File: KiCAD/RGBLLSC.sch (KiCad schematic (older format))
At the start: 16 parts, among them P1 PICKIT3, P2 RGB-LED-Strip, Q1 FQP30N06L, Q2 FQP30N06L, Q3 FQP30N06L, U1 PIC12F1840

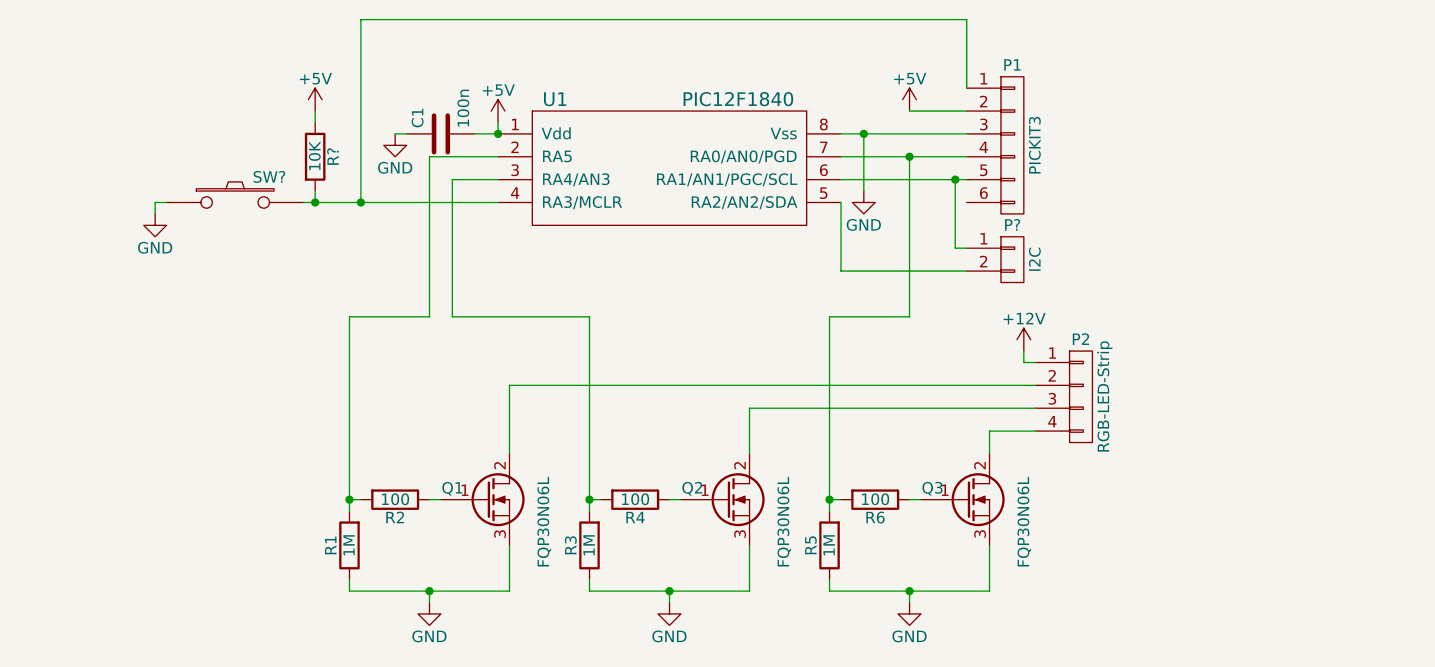
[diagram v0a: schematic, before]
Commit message: Updated Schematic
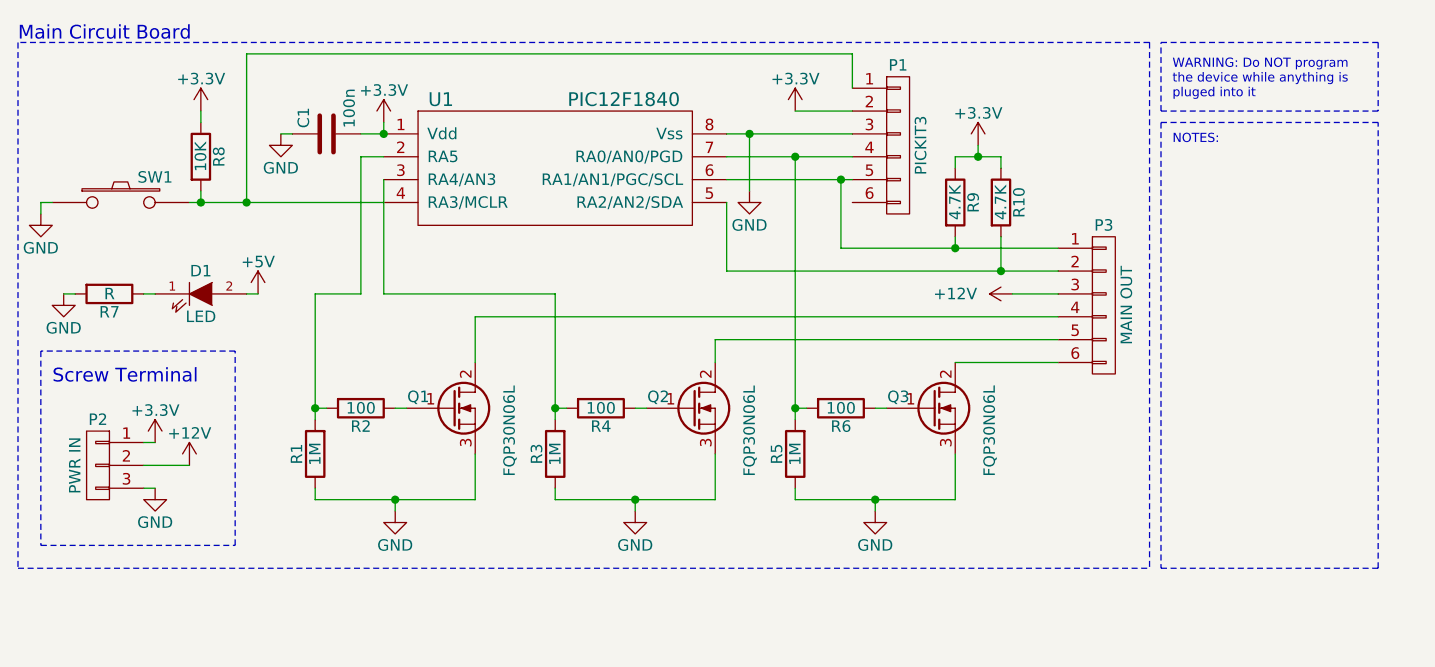
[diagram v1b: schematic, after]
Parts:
- removed P2: RGB-LED-Strip, symbol CONN_01X04
- removed P?: I2C, symbol CONN_01X02
- added D1: LED, symbol LED
- added P2: PWR IN, symbol CONN_01X03
- added P3: MAIN OUT, symbol CONN_01X06
- added R10, R9: 4.7K, symbol R
- added R7: R, symbol R
- gave numbers to parts that had none: 2
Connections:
- net +12V: now also P2.2 (P2), P3.3 (P3)
- net +5V: now also D1.2 (A); no longer C1.2, P1.2 (P2), R8.1, U1.1 (Vdd)
- net GND: now also P2.3 (P3), R7.2
- net at Q2.2 (D): now also P3.5 (P5)
- net at U1.5 (RA2/AN2/SDA): now also P3.2 (P2), R10.2
- net at P1.5 (P5), U1.6 (RA1/AN1/PGC/SCL): now also P3.1 (P1), R9.2
- net at Q1.2 (D): now also P3.4 (P4)
- net at Q3.2 (D): now also P3.6 (P6)
- new net: D1.1 (K), R7.1
- new net +3V3: C1.2, P1.2 (P2), P2.1 (P1), R10.1, R8.1, R9.1, U1.1 (Vdd)
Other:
- note added: "Main Circuit Board"
- note added: "NOTES:"
- note added: "Screw Terminal\n"
- note added: "WARNING: Do NOT program \nthe device while anything is \npluged into it"
- moved on the sheet: C1, P1, Q1, Q2, Q3, R1, R2, R3, R4, R5, R6, R8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
